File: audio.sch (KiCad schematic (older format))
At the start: 0 parts

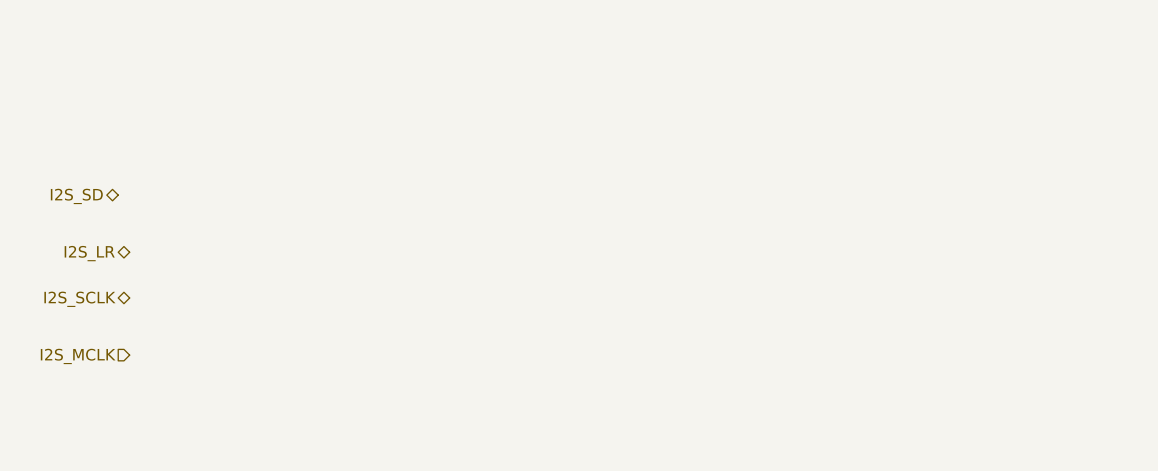
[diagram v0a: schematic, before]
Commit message: 20191114
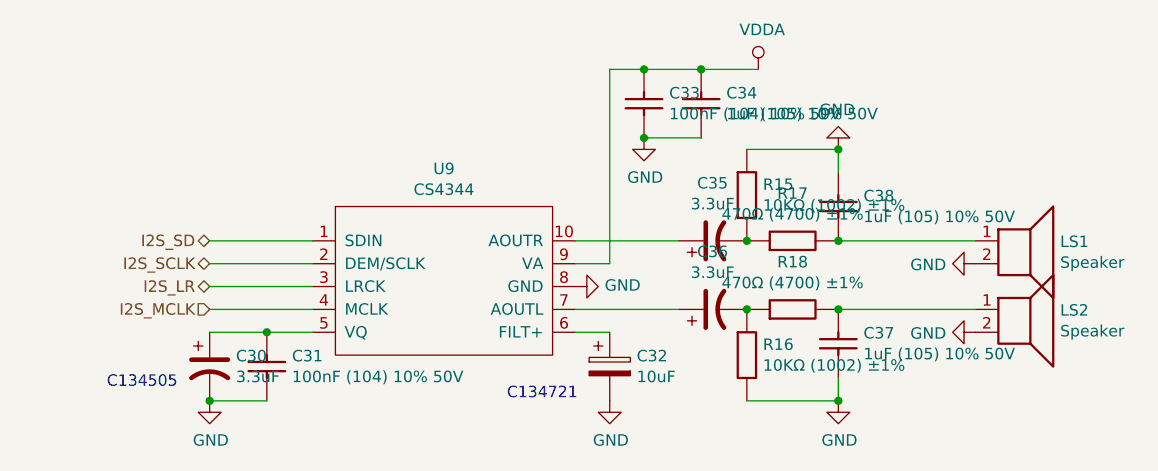
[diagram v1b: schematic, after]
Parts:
- added C30, C35, C36: 3.3uF, Capacitor_SMD:CP_Elec_4x5.4, symbol Device:CP1
- added C31, C33: 0603_100nF__104_10%_50V, lc_lib:0603_C, symbol lc_Cap:0603_100nF__104_10%_50V
- added C32: 10uF, Capacitor_SMD:CP_Elec_4x5.3, symbol Device:CP
- added C34, C37, C38: 0603_1uF__105_10%_50V, lc_lib:0603_C, symbol lc_Cap:0603_1uF__105_10%_50V
- added LS1, LS2: Speaker, Connector_PinHeader_2.54mm:PinHeader_1x02_P2.54mm_Vertical, symbol Device:Speaker
- added R15, R16: 0603_10KΩ__1002_1%, lc_lib:0603_R, symbol lc_RES:0603_10KΩ__1002_1%
- added R17, R18: 0603_470Ω__4700_1%, lc_lib:0603_R, symbol lc_RES:0603_470Ω__4700_1%
- added U9: CS4344, Package_SO:TSSOP-10_3x3mm_P0.5mm, symbol CS4344:CS4344
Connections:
- net I2S_LR: now also U9.3 (LRCK)
- net I2S_MCLK: now also U9.4 (MCLK)
- net I2S_SCLK: now also U9.2 (DEM/SCLK)
- net I2S_SD: now also U9.1 (SDIN)
- new net: C35.1, U9.10 (AOUTR)
- new net: C30.1, C31.1, U9.5 (VQ)
- new net: C32.1, U9.6 (FILT+)
- new net: C36.1, U9.7 (AOUTL)
- new net: C35.2, R15.2, R17.1
- new net: C36.2, R16.1, R18.1
- new net: C38.1, LS1.1, R17.2
- new net: C37.1, LS2.1, R18.2
- new net GND: C30.2, C31.2, C32.2, C33.2, C34.2, C37.2, C38.2, LS1.2, LS2.2, R15.1, R16.2, U9.8 (GND)
- new net VDDA: C33.1, C34.1, U9.9 (VA)
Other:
- note added: "C134505"
- note added: "C134721"
